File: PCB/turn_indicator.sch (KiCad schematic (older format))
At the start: 15 parts

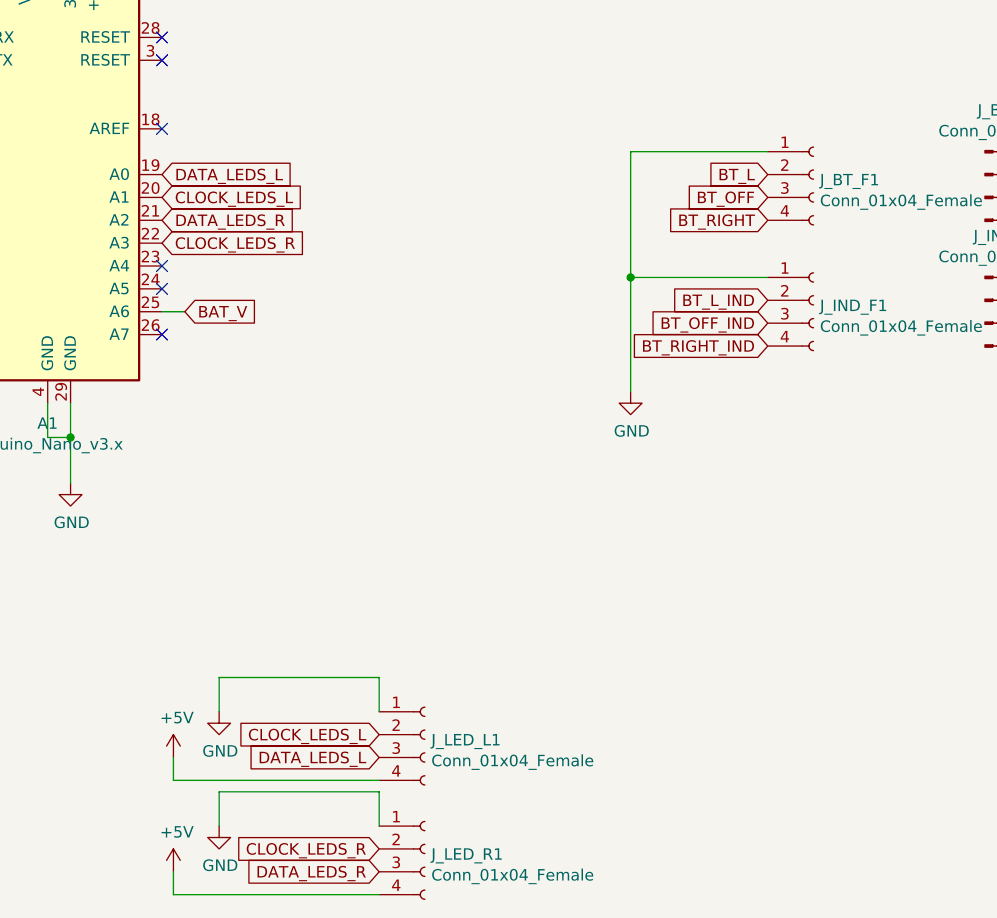
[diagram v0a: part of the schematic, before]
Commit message: pcb subfolder and unknown pending changes
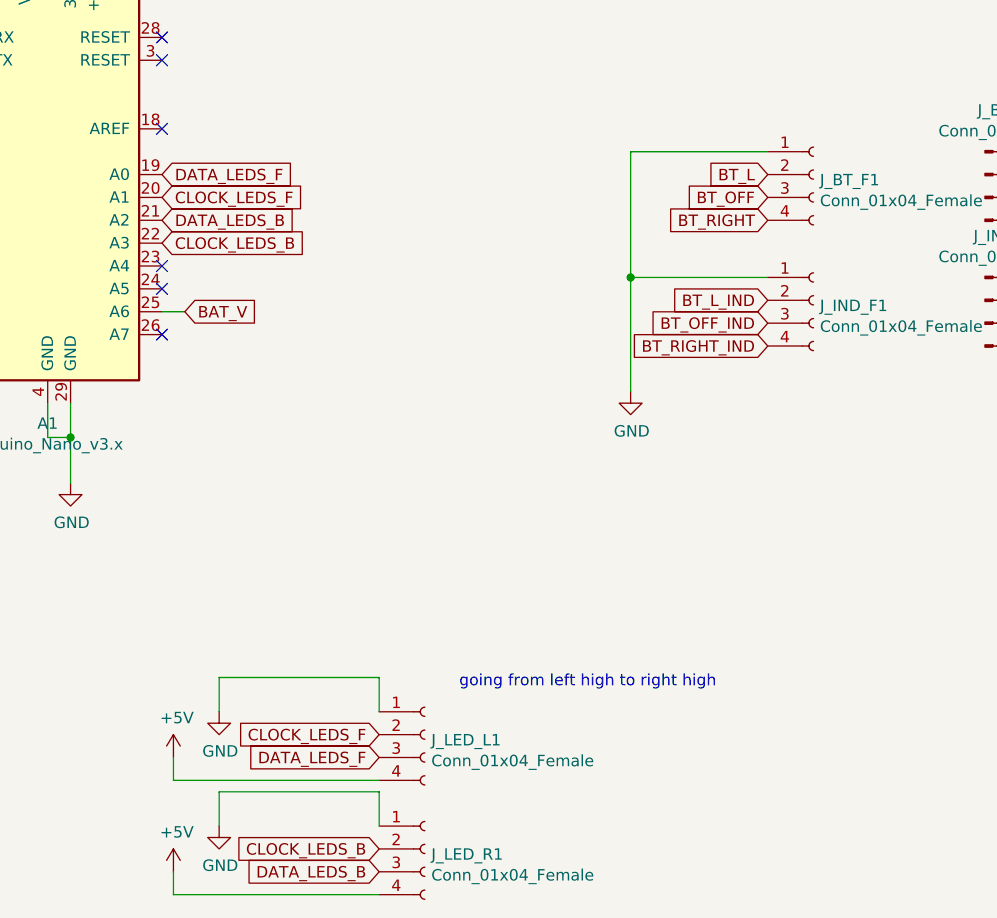
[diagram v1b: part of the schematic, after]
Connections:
- net CLOCK_LEDS_L renamed CLOCK_LEDS_F
- net CLOCK_LEDS_R renamed CLOCK_LEDS_B
- net DATA_LEDS_L renamed DATA_LEDS_F
- net DATA_LEDS_R renamed DATA_LEDS_B
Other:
- note added: "going from left high to right high"
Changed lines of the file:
@@
 PWR_IND
 Text GLabel 3950 3800 2    50   Input ~ 0
-DATA_LEDS_L
+DATA_LEDS_F
 Text GLabel 3950 3900 2    50   Input ~ 0
-CLOCK_LEDS_L
+CLOCK_LEDS_F
 $Comp
 L Connector:Conn_01x02_Male J_LIPO_SW_M1
@@
 $EndComp
 Text GLabel 4900 6850 0    50   Input ~ 0
-DATA_LEDS_R
+DATA_LEDS_B
 Text GLabel 4900 6750 0    50   Input ~ 0
-CLOCK_LEDS_R
+CLOCK_LEDS_B
 Wire Wire Line
 	4900 6500 4900 6650
 Text GLabel 4900 6350 0    50   Input ~ 0
-DATA_LEDS_L
+DATA_LEDS_F
 Text GLabel 4900 6250 0    50   Input ~ 0
-CLOCK_LEDS_L
+CLOCK_LEDS_F
 Wire Wire Line
 	4200 6000 4900 6000
@@
 $EndComp
 Text GLabel 3950 4000 2    50   Input ~ 0
-DATA_LEDS_R
+DATA_LEDS_B
 Text GLabel 3950 4100 2    50   Input ~ 0
-CLOCK_LEDS_R
+CLOCK_LEDS_B
 Wire Wire Line
 	5450 1350 5450 1450
@@
 Wire Wire Line
 	6850 1400 6850 1350
+Text Notes 5250 6050 0    50   ~ 0
+going from left high to right high
 $EndSCHEMATC
